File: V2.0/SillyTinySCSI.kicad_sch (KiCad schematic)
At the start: 24 parts, among them J1 DB25_Plug, U1 74LVT125, U2 74LVT245, U3 74LVT125, U4 74LVT245

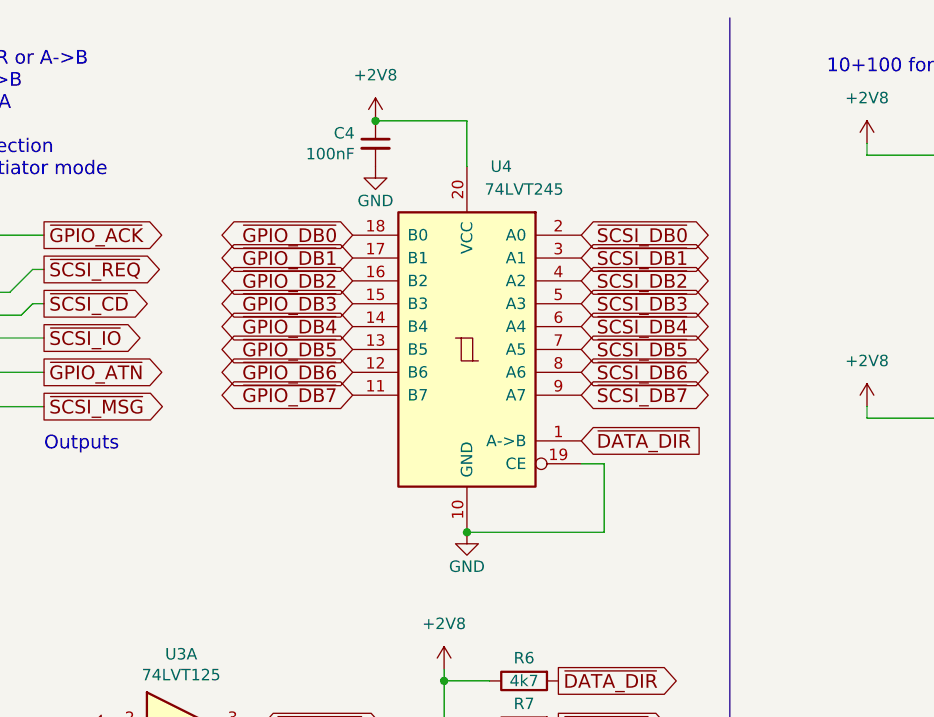
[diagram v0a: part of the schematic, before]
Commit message: last resistor pack
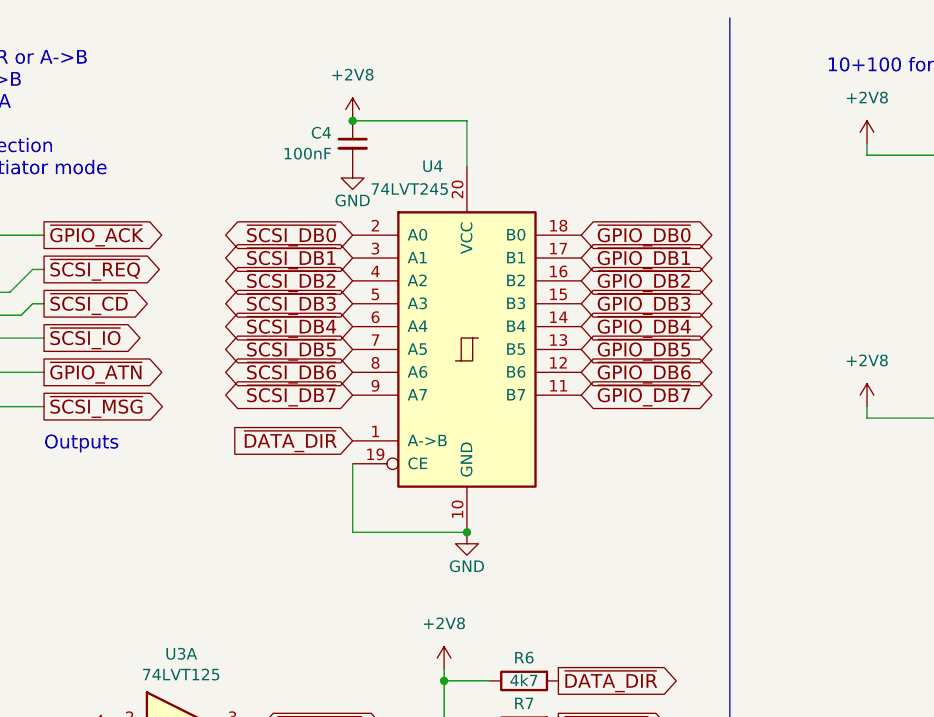
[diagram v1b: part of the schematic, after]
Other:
- moved on the sheet: C4
